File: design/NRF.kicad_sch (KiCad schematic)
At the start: 18 parts, among them J2 Conn_Coaxial, U4 nRF24L01P, X2 16MHz

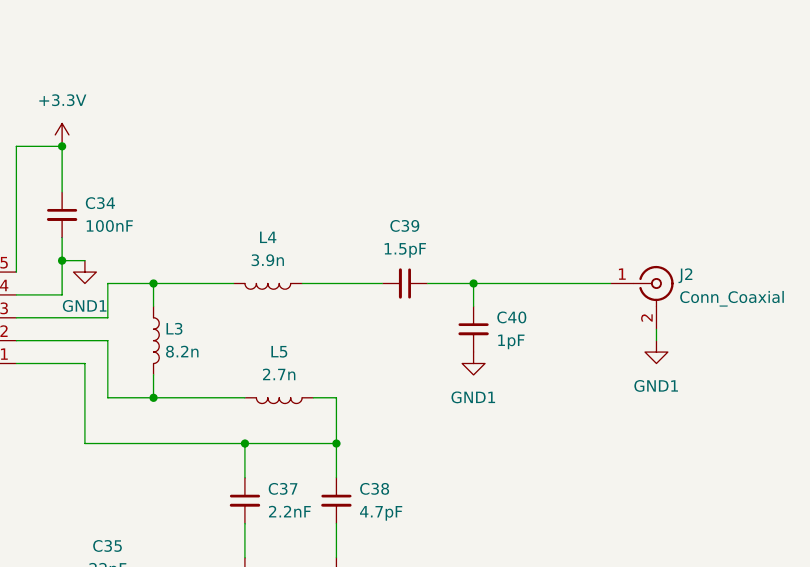
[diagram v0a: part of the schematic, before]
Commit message: Agrego MFR# de conectores
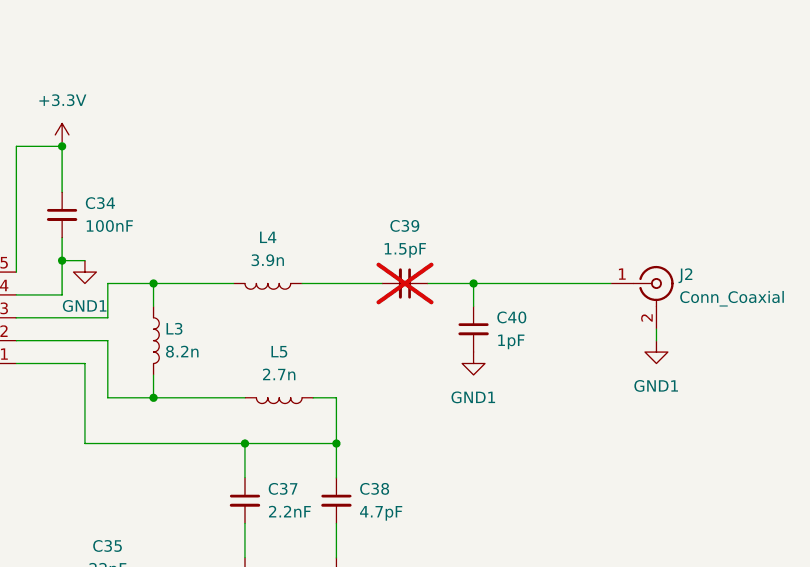
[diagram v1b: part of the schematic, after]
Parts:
- C39: now not fitted
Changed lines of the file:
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@@
 		(in_bom yes)
 		(on_board yes)
-		(dnp no)
+		(dnp yes)
 		(fields_autoplaced yes)
 		(property "Reference" "C39"
